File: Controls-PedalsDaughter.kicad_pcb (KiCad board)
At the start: 2 copper layers, 51.3 x 75 mm, 54 parts, among them J1 Brake Pos. Sensor, J2 Accel Pos. Sensor, J3 PeripheralCANConnector, J4 Conn_01x02, J5 PeripheralCANConnector, U1 RI3-1205S, U2 PeripheralSOM, U3 TLV9301xDCK, U4 TLV70130DBVR, U5 AMC1300BDWV, U6 TLV9301xDCK

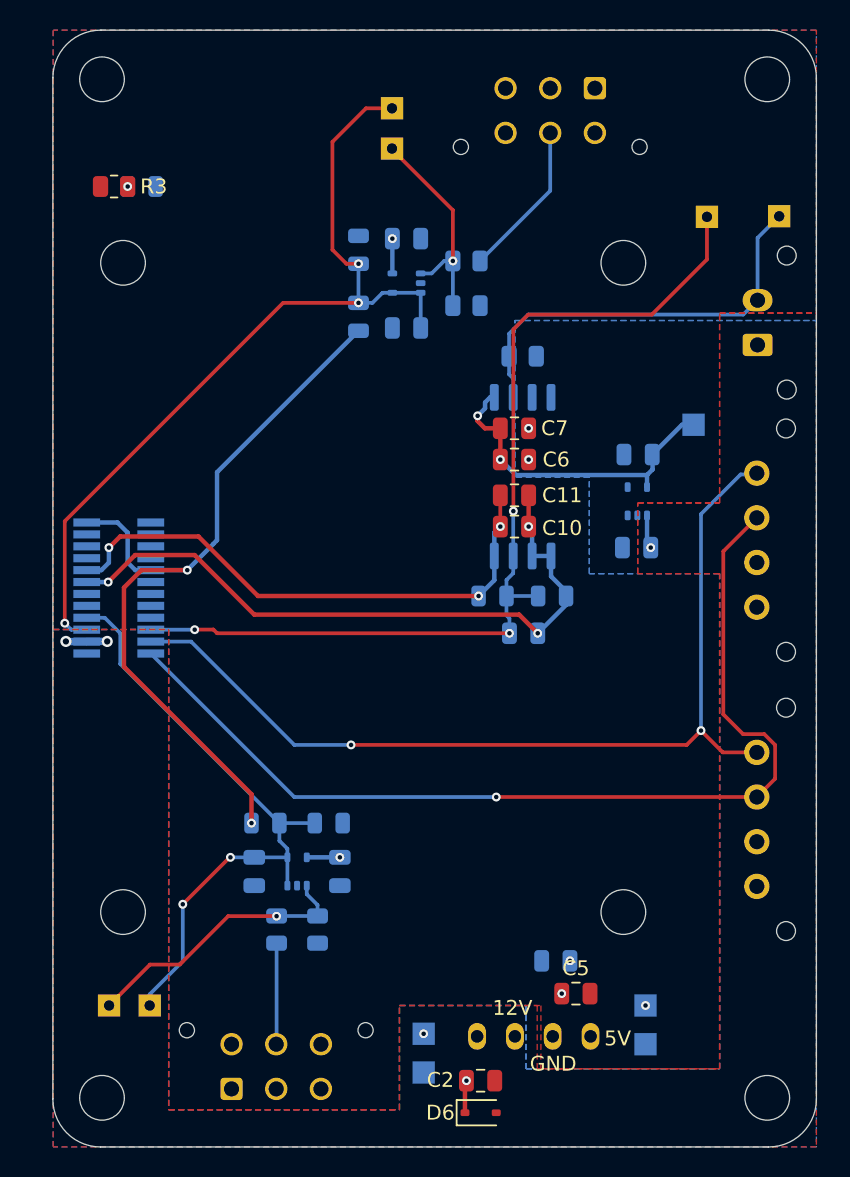
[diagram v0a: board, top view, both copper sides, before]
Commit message: new constraints
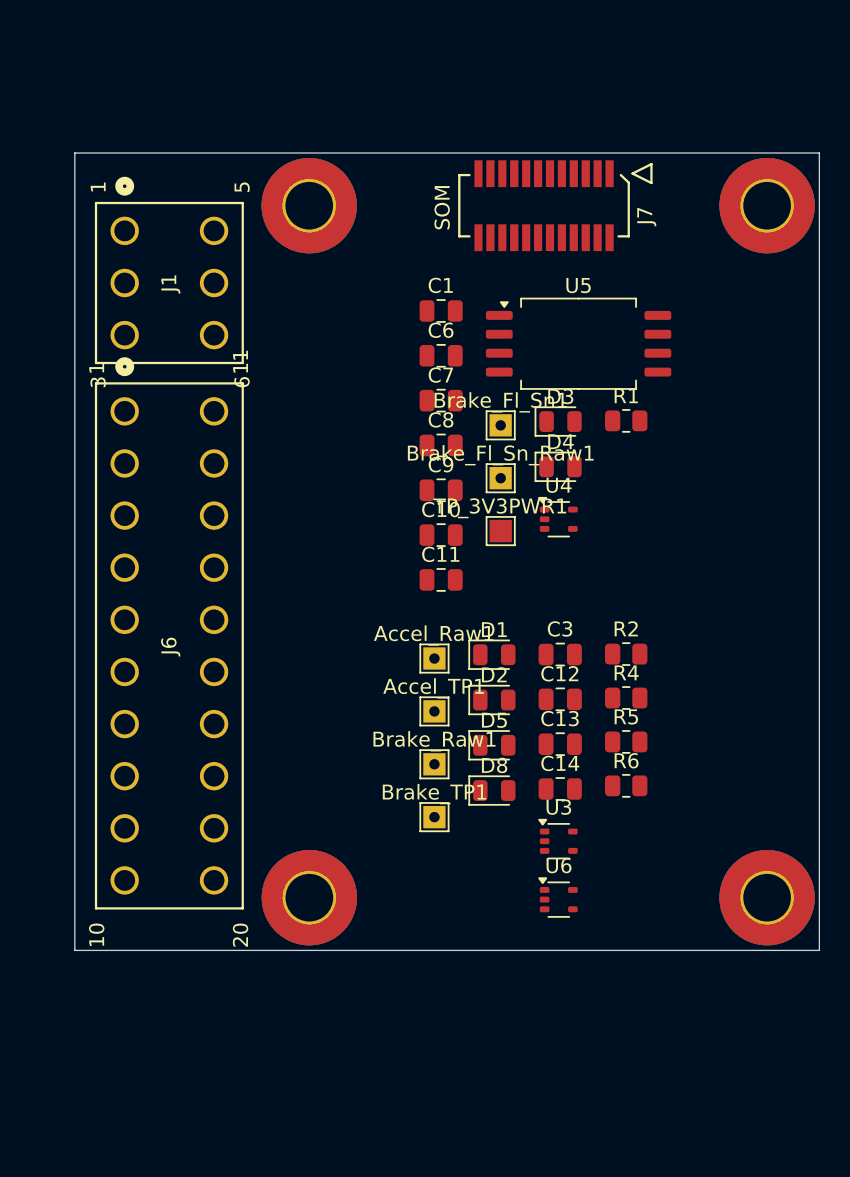
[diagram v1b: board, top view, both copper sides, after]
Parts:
- removed +12V: +12V_TP, TestPoint:TestPoint_Pad_1.5x1.5mm
- removed +5V: +5V_TP, TestPoint:TestPoint_Pad_1.5x1.5mm
- removed 3V3PWR: +3V3PWR, TestPoint:TestPoint_Pad_1.5x1.5mm
- removed ?: , clipboard:1102f6bf-9d39-4637-903a-16b78c874ac5
- removed Accel: Accel, TestPoint:TestPoint_THTPad_1.5x1.5mm_Drill0.7mm
- removed Accel_Raw: Accel_Raw_TP, TestPoint:TestPoint_THTPad_1.5x1.5mm_Drill0.7mm
- removed Brake: Brake, TestPoint:TestPoint_THTPad_1.5x1.5mm_Drill0.7mm
- removed Brake_Fl: Brake_Fl_Sn_TP, TestPoint:TestPoint_THTPad_1.5x1.5mm_Drill0.7mm
- removed Brake_Fl_Raw: Brake_Fl_Sn_Raw_TP, TestPoint:TestPoint_THTPad_1.5x1.5mm_Drill0.7mm
- removed Brake_Raw: Brake_Raw_TP, TestPoint:TestPoint_THTPad_1.5x1.5mm_Drill0.7mm
- removed C2: 10uF, Capacitor_SMD:C_0805_2012Metric
- removed C4: 10uf, Capacitor_SMD:C_0805_2012Metric
- removed C5: .1uf, Capacitor_SMD:C_0805_2012Metric
- removed D6: PESD15VL1BA, Diode_SMD:D_SOD-323
- removed GND: GND_TP, TestPoint:TestPoint_Pad_1.5x1.5mm
- removed GNDPWR: GNDPWR_TP, TestPoint:TestPoint_Pad_1.5x1.5mm
- removed H1, H2, H3: MountingHole, clipboard:1102f6bf-9d39-4637-903a-16b78c874ac5
- removed J2: Accel Pos. Sensor, Connector_Molex:Molex_Micro-Fit_3.0_43045-0612_2x03_P3.00mm_Vertical
- removed J3, J5: PeripheralCANConnector, UTSVT_Connectors:Molex_MicroFit3.0_1x4xP3.00mm_PolarizingPeg_Vertical
- removed J4: Conn_01x02, Connector_Molex:Molex_Micro-Fit_3.0_43650-0215_1x02_P3.00mm_Vertical
- removed PWR: SMD_0805, Diode_SMD:D_0805_2012Metric
- removed R3: 1.5k, Resistor_SMD:R_0805_2012Metric
- removed U1: RI3-1205S, UTSVT_ICs:RI3_DC_Converter
- removed U2: PeripheralSOM, UTSVT_Special:PeripheralSOM
- added Accel_Raw1: Accel_Raw_TP, TestPoint:TestPoint_THTPad_1.5x1.5mm_Drill0.7mm, F.Cu at (148.1, 104.7)
- added Accel_TP1: Accel, TestPoint:TestPoint_THTPad_1.5x1.5mm_Drill0.7mm, F.Cu at (148.1, 108.2)
- added Brake_Fl_Sn1: Brake_Fl_Sn_TP, TestPoint:TestPoint_THTPad_1.5x1.5mm_Drill0.7mm, F.Cu at (152.6, 89.0)
- added Brake_Fl_Sn_Raw1: Brake_Fl_Sn_Raw_TP, TestPoint:TestPoint_THTPad_1.5x1.5mm_Drill0.7mm, F.Cu at (152.6, 92.6)
- added Brake_Raw1: Brake_Raw_TP, TestPoint:TestPoint_THTPad_1.5x1.5mm_Drill0.7mm, F.Cu at (148.1, 111.8)
- added Brake_TP1: Brake, TestPoint:TestPoint_THTPad_1.5x1.5mm_Drill0.7mm, F.Cu at (148.1, 115.3)
- added J6: MX150_02x10_Vertical, UTSVT_Connectors:CONN_SD-75757-002_2X10_F16p09_MOL, F.Cu at (130.3, 103.8)
- added J7: 53307-2471, UTSVT_Connectors:PeripheralSOM, F.Cu at (155.5, 74.3)
- added TP_3V3PWR1: +3V3PWR, TestPoint:TestPoint_Pad_1.5x1.5mm, F.Cu at (152.6, 96.1)
- C1, C12, C13, C14, C3, C8, C9, D1, D2, D3, D4, D5, D8, R1, R2, R4, R5, R6, U3, U4, U5, U6: moved to F.Cu
- J1: value Brake Pos. Sensor -> MX150_02x03_Vertical; footprint Connector_Molex:Molex_Micro-Fit_3.0_43045-0612_2x03_P3.00mm_Vertical -> UTSVT_Connectors:CONN06_0757575131_MOL; moved to F.Cu
- moved U6 42.6 mm to (156.4, 120.9), turned to 0 degrees
- moved D8 37.4 mm to (152.1, 113.6), turned to 0 degrees
- moved C13 35.5 mm to (156.6, 110.5), turned to 0 degrees
- moved R5 34.0 mm to (161.0, 110.3)
- moved R6 34.0 mm to (161.0, 113.2)
- moved C14 32.6 mm to (156.6, 113.5)
- moved J1 31.4 mm to (130.3, 79.5), turned to 90 degrees
- moved D5 30.2 mm to (152.1, 110.5), turned to 0 degrees
- moved R2 29.9 mm to (161.0, 104.4), turned to 0 degrees
- moved R4 25.9 mm to (161.0, 107.3), turned to 0 degrees
- moved C12 23.6 mm to (156.6, 107.4), turned to 0 degrees
- moved C3 20.8 mm to (156.6, 104.4), turned to 0 degrees
- moved C1 20.6 mm to (148.6, 81.4), turned to 0 degrees
- moved D1 19.1 mm to (152.1, 104.4)
- moved U3 17.7 mm to (156.4, 117.0), turned to 0 degrees
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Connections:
- J1 pad 1: GND -> unconnected-(J1-+24V-Pad1)
- J1 pad 3: GND -> unconnected-(J1-CANL_IN-Pad3)
- J1 pad 4: +5V -> unconnected-(J1-GND-Pad4)
- J1 pad 5: Net-(J1-Pin_5) -> unconnected-(J1-CANH_OUT-Pad5)
- J1 pad 6: +5V -> unconnected-(J1-CANL_OUT-Pad6)
- R2 pad 2: Net-(J2-Pin_5) -> unconnected-(R2-Pad2)
- R5 pad 2: Net-(J1-Pin_5) -> unconnected-(R5-Pad2)
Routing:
- net /CAN_H: track 67.4 -> 0.00 mm, vias 1 -> 0
- net /Brake_Fl: track 64.8 -> 0.00 mm, vias 3 -> 0
- net /CAN_L: track 64.0 -> 0.00 mm, vias 2 -> 0
- net /Brake_Pot: track 58.1 -> 0.00 mm, vias 3 -> 0
- net +3V3: track 54.2 -> 0.00 mm, vias 2 -> 0
- net GNDA: track 45.5 -> 0.00 mm, vias 3 -> 0
- net /Accel: track 42.8 -> 0.00 mm, vias 2 -> 0
- net +VDDA: track 37.2 -> 0.00 mm, vias 3 -> 0
- net /Brake Fluid Sensor/INP: track 28.2 -> 0.00 mm
- net +3V3PWR: track 22.3 -> 0.00 mm, vias 2 -> 0
- net Net-(U3-+): track 18.8 -> 0.00 mm, vias 1 -> 0
- net Net-(U6-+): track 14.8 -> 0.00 mm, vias 1 -> 0
- net Net-(J1-Pin_5): track 11.0 -> 0.00 mm
- net Net-(J2-Pin_5): track 7.03 -> 0.00 mm
- net +12V: track 5.03 -> 0.00 mm, vias 4 -> 0
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- removed copper zone on F.Cu, net +12V
- removed copper zone on F.Cu, net +5V
- removed copper zone on B.Cu, net GND
- removed copper zone on B.Cu, net GNDPWR
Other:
- board size 51.3 x 75 mm -> 50 x 53.5 mm
- board text removed: "+"
- board text removed: "-"
- board text removed: "12V"
- board text removed: "5V"
- board text removed: "ACC"
- board text removed: "Accel"
- board text removed: "BRK"
- board text removed: "Brake"
- board text removed: "CAN"
- board text removed: "FL_SN"
- board text removed: "GND"
- board text removed: "GP"
- board text removed: "H"
- board text removed: "IN"
- board text removed: "L"
- board text removed: "This area needs to be clear for USBC"

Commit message: update
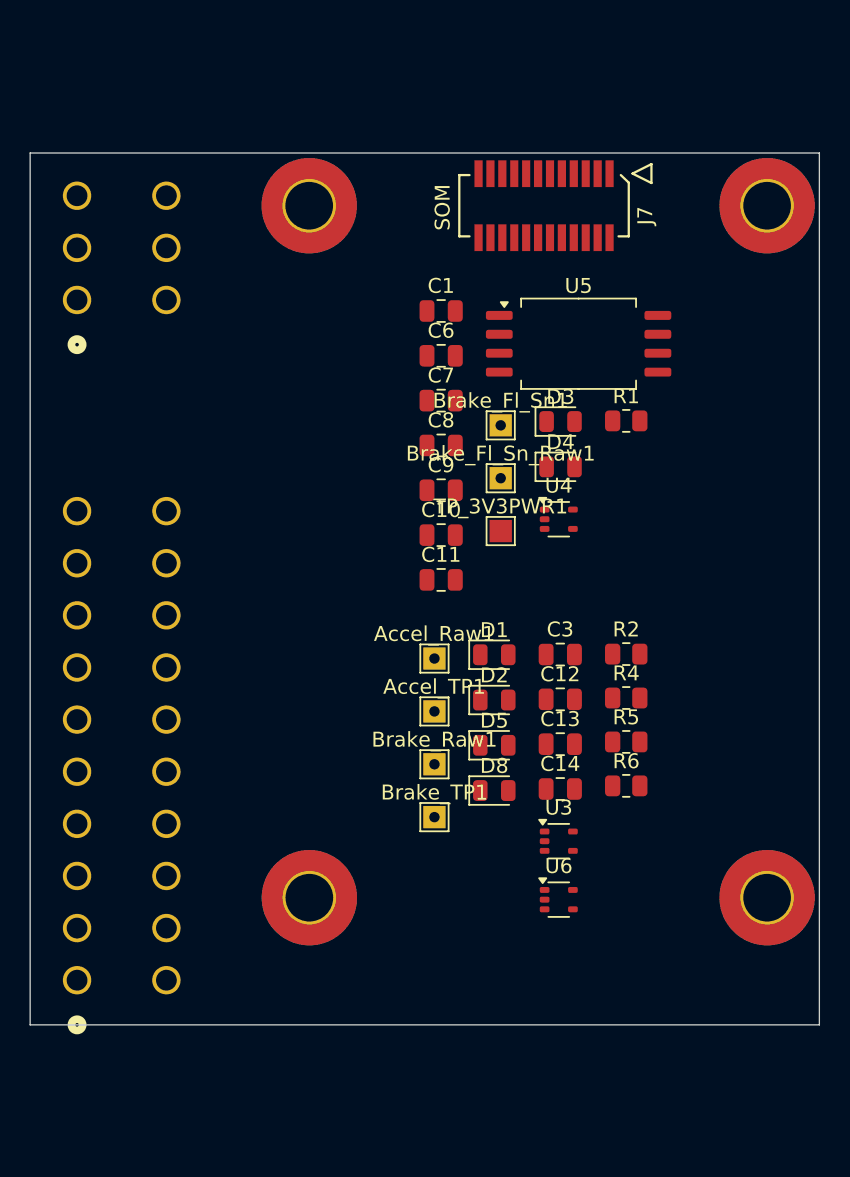
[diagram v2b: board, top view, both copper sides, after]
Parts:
- J1, J6: moved to B.Cu
- moved J6 7.61 mm to (127.1, 110.6), turned to -90 degrees
- moved J1 3.98 mm to (127.1, 77.1), turned to -90 degrees
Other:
- board size 50 x 53.5 mm -> 53 x 58.6 mm
